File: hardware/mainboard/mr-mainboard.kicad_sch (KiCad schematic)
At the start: 0 parts

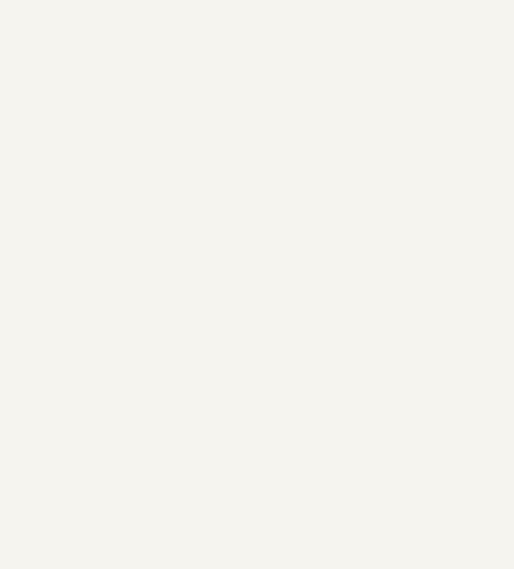
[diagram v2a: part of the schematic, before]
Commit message: Working on layout
Signed-off-by: David Shah <dave@ds0.me>
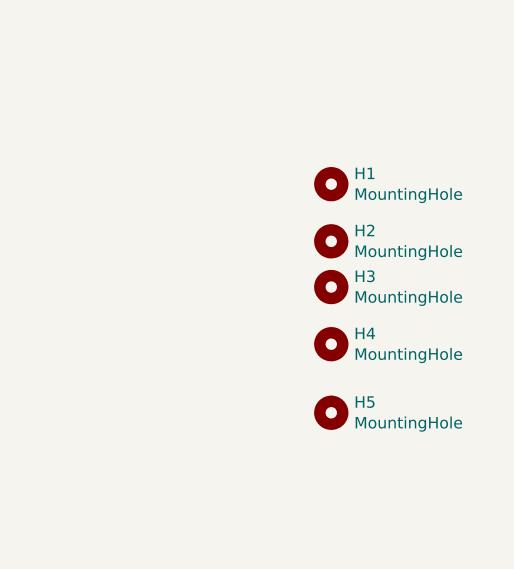
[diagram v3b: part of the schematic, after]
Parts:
- added H1, H2, H3, H4: MountingHole, MountingHole:MountingHole_2.7mm_M2.5, symbol Mechanical:MountingHole
- added H5: MountingHole, meowality:9774025151R, symbol Mechanical:MountingHole
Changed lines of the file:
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@@
 (kicad_sch (version 20210126) (generator eeschema)
   (paper "A4")
+  (symbol (lib_id "Mechanical:MountingHole") (at 215.9 63.5 0) (unit 1)
+    (in_bom yes) (on_board yes)
+    (property "Reference" "H1" (id 0) (at 218.4401 62.3506 0)
+      (effects (font (size 1.27 1.27)) (justify left))
+    )
+    (property "Value" "MountingHole" (id 1) (at 218.4401 64.6493 0)
+      (effects (font (size 1.27 1.27)) (justify left))
+    )
+    (property "Footprint" "MountingHole:MountingHole_2.7mm_M2.5" (id 2) (at 215.9 63.5 0)
+      (effects (font (size 1.27 1.27)) hide)
+    )
+    (property "Datasheet" "~" (id 3) (at 215.9 63.5 0)
+      (effects (font (size 1.27 1.27)) hide)
+    )
+  )
+  (symbol (lib_id "Mechanical:MountingHole") (at 215.9 69.85 0) (unit 1)
+    (in_bom yes) (on_board yes)
+    (property "Reference" "H2" (id 0) (at 218.4401 68.7006 0)
+      (effects (font (size 1.27 1.27)) (justify left))
+    )
+    (property "Value" "MountingHole" (id 1) (at 218.4401 70.9993 0)
+      (effects (font (size 1.27 1.27)) (justify left))
+    )
+    (property "Footprint" "MountingHole:MountingHole_2.7mm_M2.5" (id 2) (at 215.9 69.85 0)
+      (effects (font (size 1.27 1.27)) hide)
+    )
+    (property "Datasheet" "~" (id 3) (at 215.9 69.85 0)
+      (effects (font (size 1.27 1.27)) hide)
+    )
+  )
+  (symbol (lib_id "Mechanical:MountingHole") (at 215.9 74.93 0) (unit 1)
+    (in_bom yes) (on_board yes)
+    (property "Reference" "H3" (id 0) (at 218.4401 73.7806 0)
+      (effects (font (size 1.27 1.27)) (justify left))
+    )
+    (property "Value" "MountingHole" (id 1) (at 218.4401 76.0793 0)
+      (effects (font (size 1.27 1.27)) (justify left))
+    )
+    (property "Footprint" "MountingHole:MountingHole_2.7mm_M2.5" (id 2) (at 215.9 74.93 0)
+      (effects (font (size 1.27 1.27)) hide)
+    )
+    (property "Datasheet" "~" (id 3) (at 215.9 74.93 0)
+      (effects (font (size 1.27 1.27)) hide)
+    )
+  )
+  (symbol (lib_id "Mechanical:MountingHole") (at 215.9 81.28 0) (unit 1)
+    (in_bom yes) (on_board yes)
+    (property "Reference" "H4" (id 0) (at 218.4401 80.1306 0)
+      (effects (font (size 1.27 1.27)) (justify left))
+    )
+    (property "Value" "MountingHole" (id 1) (at 218.4401 82.4293 0)
+      (effects (font (size 1.27 1.27)) (justify left))
+    )
+    (property "Footprint" "MountingHole:MountingHole_2.7mm_M2.5" (id 2) (at 215.9 81.28 0)
+      (effects (font (size 1.27 1.27)) hide)
+    )
+    (property "Datasheet" "~" (id 3) (at 215.9 81.28 0)
+      (effects (font (size 1.27 1.27)) hide)
+    )
+  )
+  (symbol (lib_id "Mechanical:MountingHole") (at 215.9 88.9 0) (unit 1)
+    (in_bom yes) (on_board yes)
+    (property "Reference" "H5" (id 0) (at 218.4401 87.7506 0)
+      (effects (font (size 1.27 1.27)) (justify left))
+    )
+    (property "Value" "MountingHole" (id 1) (at 218.4401 90.0493 0)
+      (effects (font (size 1.27 1.27)) (justify left))
+    )
+    (property "Footprint" "meowality:9774025151R" (id 2) (at 215.9 88.9 0)
+      (effects (font (size 1.27 1.27)) hide)
+    )
+    (property "Datasheet" "~" (id 3) (at 215.9 88.9 0)
+      (effects (font (size 1.27 1.27)) hide)
+    )
+  )
   (sheet (at 114.3 38.1) (size 25.4 25.4)
     (stroke (width 0.001) (type solid) (color 132 0 132 1))
@@
   )
   (symbol_instances
+    (path "/2a727066-23b2-42f4-88da-4f7a020b89b2"
+      (reference "H1") (unit 1) (value "MountingHole") (footprint "MountingHole:MountingHole_2.7mm_M2.5")
+    )
+    (path "/fc4ecb81-0f51-4040-adf5-7e03fcfc8710"
+      (reference "H2") (unit 1) (value "MountingHole") (footprint "MountingHole:MountingHole_2.7mm_M2.5")
+    )
+    (path "/710b30eb-77ed-4d74-a17c-e1969039ca62"
+      (reference "H3") (unit 1) (value "MountingHole") (footprint "MountingHole:MountingHole_2.7mm_M2.5")
+    )
+    (path "/39218fa2-549f-495c-977f-2517a7785a2b"
+      (reference "H4") (unit 1) (value "MountingHole") (footprint "MountingHole:MountingHole_2.7mm_M2.5")
+    )
+    (path "/a5d91f34-d2a0-4453-93ad-825a450a8ddb"
+      (reference "H5") (unit 1) (value "MountingHole") (footprint "meowality:9774025151R")
+    )
     (path "/7dd540ee-d364-4396-a5ce-94105f298dc9/4dd6052b-4c44-4337-bca1-1febcef57c4e"
       (reference "#PWR01") (unit 1) (value "GND") (footprint "")
@@
     )
     (path "/fab76c53-3adb-4867-b007-ffb14aef2f22/1f28fc80-5e32-4c90-8262-fb490a2e71b9"
-      (reference "J3") (unit 1) (value "EAR") (footprint "Connector_PinHeader_2.54mm:PinHeader_2x03_P2.54mm_Horizontal")
+      (reference "J3") (unit 1) (value "EAR") (footprint "Connector_PinHeader_2.00mm:PinHeader_2x03_P2.00mm_Horizontal")
     )
     (path "/fab76c53-3adb-4867-b007-ffb14aef2f22/03adfbf0-11f4-4773-98d0-8b49bcac8472"
@@
       (reference "R26") (unit 1) (value "10k") (footprint "Resistor_SMD:R_0402_1005Metric")
     )
-    (path "/fab76c53-3adb-4867-b007-ffb14aef2f22/b0efb6e7-77d4-48b3-90d5-8ce2ee293e5d"
-      (reference "R27") (unit 1) (value "10k") (footprint "Resistor_SMD:R_0402_1005Metric")
-    )
     (path "/fab76c53-3adb-4867-b007-ffb14aef2f22/66fe7f9b-8d05-4724-aaa2-93952a700c19"
       (reference "R28") (unit 1) (value "10k") (footprint "Resistor_SMD:R_0402_1005Metric")
@@
       (reference "SW1") (unit 1) (value "SW_Push") (footprint "Button_Switch_THT:SW_Tactile_SPST_Angled_PTS645Vx31-2LFS")
     )
-    (path "/fab76c53-3adb-4867-b007-ffb14aef2f22/11249cce-8d50-4594-ac41-e1138b1e2a24"
+    (path "/fab76c53-3adb-4867-b007-ffb14aef2f22/7334a4b3-93c3-48c5-b0b3-231670f445fd"
       (reference "SW2") (unit 1) (value "SW_Push") (footprint "Button_Switch_THT:SW_Tactile_SPST_Angled_PTS645Vx31-2LFS")
     )
-    (path "/fab76c53-3adb-4867-b007-ffb14aef2f22/7334a4b3-93c3-48c5-b0b3-231670f445fd"
-      (reference "SW3") (unit 1) (value "SW_Push") (footprint "Button_Switch_THT:SW_Tactile_SPST_Angled_PTS645Vx31-2LFS")
-    )
     (path "/fab76c53-3adb-4867-b007-ffb14aef2f22/5ef466bb-b771-4c4a-8164-fe0f34a373fa"
